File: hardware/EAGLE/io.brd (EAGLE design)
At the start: 17.8 x 110.5 mm, 23 parts, among them J10 PJ301_THONKICONN6, J11 PJ301_THONKICONN6, J12 PJ301_THONKICONN6, J13 PJ301_THONKICONN6, J2 PJ301_THONKICONN6, J3 PJ301_THONKICONN6, J4 PJ301_THONKICONN6, J5 PJ301_THONKICONN6, J6 PJ301_THONKICONN6, J7 PJ301_THONKICONN6, J8 PJ301_THONKICONN6, J9 PJ301_THONKICONN6

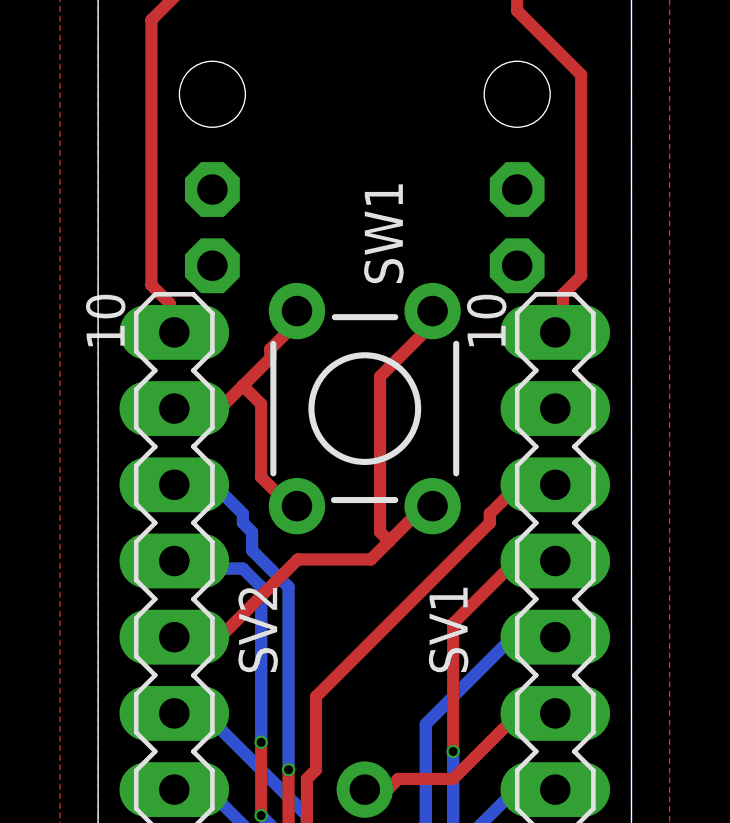
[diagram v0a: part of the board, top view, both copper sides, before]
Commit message: Submitted for Artist
and quick fixed layer errors
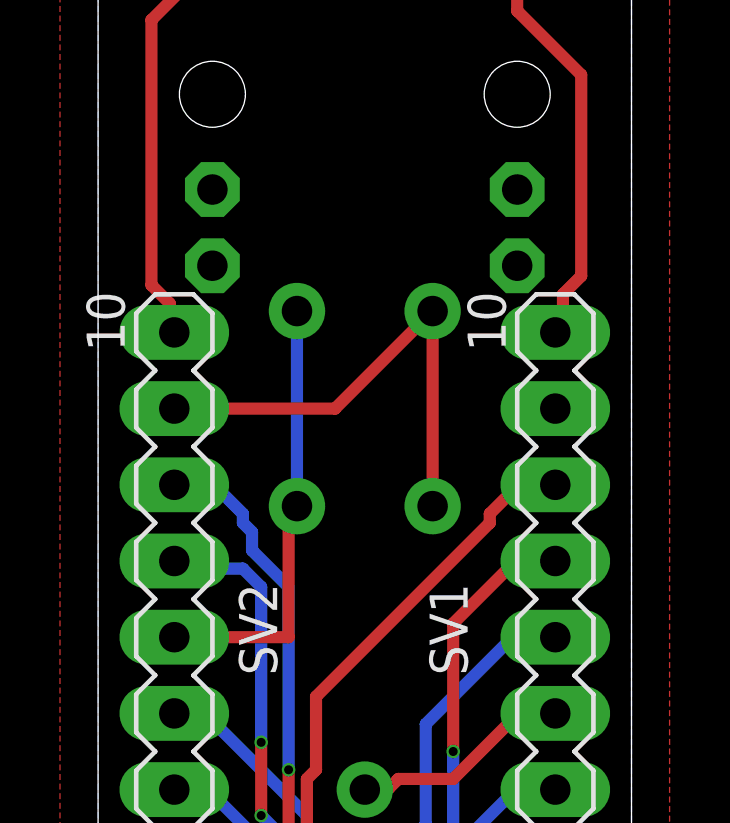
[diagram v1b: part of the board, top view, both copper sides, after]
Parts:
- flipped SW1 to the bottom
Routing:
- net +12V: track 10.8 -> 16.3 mm
- net BUTTON: track 19.1 -> 14.8 mm
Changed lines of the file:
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@@
 <attribute name="VALUE" x="13.97" y="14.351" size="1.27" layer="27" ratio="10" rot="R180"/>
 </element>
-<element name="SW1" library="SparkFun" package="TACTILE-PTH" value="" x="10.16" y="102.87" smashed="yes" rot="R90">
-<attribute name="NAME" x="10.16" y="110.49" size="1.27" layer="25" ratio="10" rot="R270"/>
+<element name="SW1" library="SparkFun" package="TACTILE-PTH" value="" x="10.16" y="102.87" smashed="yes" rot="MR90">
+<attribute name="NAME" x="10.16" y="110.49" size="1.27" layer="26" ratio="10" rot="MR270"/>
 </element>
 </elements>
@@
 <contactref element="SW1" pad="4"/>
 <contactref element="SW1" pad="3"/>
-<wire x1="5.4864" y1="95.4024" x2="3.9624" y2="95.4024" width="0.4064" layer="1"/>
-<wire x1="7.9248" y1="97.8408" x2="5.4864" y2="95.4024" width="0.4064" layer="1"/>
-<wire x1="10.3632" y1="97.8408" x2="7.9248" y2="97.8408" width="0.4064" layer="1"/>
-<wire x1="12.192" y1="99.6696" x2="10.9728" y2="98.4504" width="0.4064" layer="1"/>
-<wire x1="10.9728" y1="98.4504" x2="10.3632" y2="97.8408" width="0.4064" layer="1"/>
-<wire x1="3.9624" y1="95.4024" x2="3.81" y2="95.25" width="0.4064" layer="1"/>
-<wire x1="12.192" y1="99.6696" x2="12.4206" y2="99.6188" width="0.4064" layer="1"/>
-<wire x1="12.192" y1="105.4608" x2="12.192" y2="106.0704" width="0.4064" layer="1"/>
-<wire x1="10.668" y1="103.9368" x2="12.192" y2="105.4608" width="0.4064" layer="1"/>
-<wire x1="10.668" y1="98.7552" x2="10.668" y2="103.9368" width="0.4064" layer="1"/>
-<wire x1="10.9728" y1="98.4504" x2="10.668" y2="98.7552" width="0.4064" layer="1"/>
-<wire x1="12.192" y1="106.0704" x2="12.4206" y2="106.1212" width="0.4064" layer="1"/>
+<wire x1="7.8994" y1="99.6188" x2="7.62" y2="99.3394" width="0.4064" layer="1"/>
+<wire x1="7.62" y1="99.3394" x2="7.62" y2="95.25" width="0.4064" layer="1"/>
+<wire x1="7.62" y1="95.25" x2="3.81" y2="95.25" width="0.4064" layer="1"/>
+<wire x1="7.8994" y1="106.1212" x2="7.8994" y2="99.6188" width="0.4064" layer="16"/>
 </signal>
 <signal name="STEP">
@@
 <contactref element="SW1" pad="1"/>
 <contactref element="SW1" pad="2"/>
-<wire x1="5.4864" y1="103.0224" x2="3.9624" y2="103.0224" width="0.4064" layer="1"/>
-<wire x1="7.0104" y1="104.5464" x2="6.096" y2="103.632" width="0.4064" layer="1"/>
-<wire x1="6.096" y1="103.632" x2="5.4864" y2="103.0224" width="0.4064" layer="1"/>
-<wire x1="7.0104" y1="104.8512" x2="7.0104" y2="104.5464" width="0.4064" layer="1"/>
-<wire x1="7.62" y1="105.4608" x2="7.0104" y2="104.8512" width="0.4064" layer="1"/>
-<wire x1="7.62" y1="106.0704" x2="7.62" y2="105.4608" width="0.4064" layer="1"/>
-<wire x1="3.9624" y1="103.0224" x2="3.81" y2="102.87" width="0.4064" layer="1"/>
-<wire x1="7.62" y1="106.0704" x2="7.8994" y2="106.1212" width="0.4064" layer="1"/>
-<wire x1="6.7056" y1="100.584" x2="7.62" y2="99.6696" width="0.4064" layer="1"/>
-<wire x1="6.7056" y1="103.0224" x2="6.7056" y2="100.584" width="0.4064" layer="1"/>
-<wire x1="6.096" y1="103.632" x2="6.7056" y2="103.0224" width="0.4064" layer="1"/>
-<wire x1="7.62" y1="99.6696" x2="7.8994" y2="99.6188" width="0.4064" layer="1"/>
+<wire x1="12.4206" y1="106.1212" x2="12.2047" y2="105.9053" width="0.4064" layer="1"/>
+<wire x1="12.2047" y1="105.9053" x2="9.1694" y2="102.87" width="0.4064" layer="1"/>
+<wire x1="9.1694" y1="102.87" x2="3.81" y2="102.87" width="0.4064" layer="1"/>
+<wire x1="12.4206" y1="99.6188" x2="12.4206" y2="105.6894" width="0.4064" layer="1"/>
+<wire x1="12.4206" y1="105.6894" x2="12.2047" y2="105.9053" width="0.4064" layer="1"/>
 </signal>
 </signals>

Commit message: Added BOM
And buffer caps, and refined design
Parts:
- SV1, SV2: value (none) -> 1x10 pin header
- SV3: value (none) -> 1x3 pin header
- SW1: value (none) -> SPDT On-Off-On
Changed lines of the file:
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@@
 <layer number="25" name="tNames" color="7" fill="1" visible="yes" active="yes"/>
 <layer number="26" name="bNames" color="7" fill="1" visible="yes" active="yes"/>
-<layer number="27" name="tValues" color="7" fill="1" visible="no" active="yes"/>
-<layer number="28" name="bValues" color="7" fill="1" visible="no" active="yes"/>
-<layer number="29" name="tStop" color="7" fill="3" visible="no" active="yes"/>
-<layer number="30" name="bStop" color="7" fill="6" visible="no" active="yes"/>
-<layer number="31" name="tCream" color="7" fill="4" visible="no" active="yes"/>
-<layer number="32" name="bCream" color="7" fill="5" visible="no" active="yes"/>
-<layer number="33" name="tFinish" color="6" fill="3" visible="no" active="yes"/>
-<layer number="34" name="bFinish" color="6" fill="6" visible="no" active="yes"/>
-<layer number="35" name="tGlue" color="7" fill="4" visible="no" active="yes"/>
-<layer number="36" name="bGlue" color="7" fill="5" visible="no" active="yes"/>
-<layer number="37" name="tTest" color="7" fill="1" visible="no" active="yes"/>
-<layer number="38" name="bTest" color="7" fill="1" visible="no" active="yes"/>
+<layer number="27" name="tValues" color="7" fill="1" visible="yes" active="yes"/>
+<layer number="28" name="bValues" color="7" fill="1" visible="yes" active="yes"/>
+<layer number="29" name="tStop" color="7" fill="3" visible="yes" active="yes"/>
+<layer number="30" name="bStop" color="7" fill="6" visible="yes" active="yes"/>
+<layer number="31" name="tCream" color="7" fill="4" visible="yes" active="yes"/>
+<layer number="32" name="bCream" color="7" fill="5" visible="yes" active="yes"/>
+<layer number="33" name="tFinish" color="6" fill="3" visible="yes" active="yes"/>
+<layer number="34" name="bFinish" color="6" fill="6" visible="yes" active="yes"/>
+<layer number="35" name="tGlue" color="7" fill="4" visible="yes" active="yes"/>
+<layer number="36" name="bGlue" color="7" fill="5" visible="yes" active="yes"/>
+<layer number="37" name="tTest" color="7" fill="1" visible="yes" active="yes"/>
+<layer number="38" name="bTest" color="7" fill="1" visible="yes" active="yes"/>
 <layer number="39" name="tKeepout" color="4" fill="11" visible="yes" active="yes"/>
 <layer number="40" name="bKeepout" color="1" fill="11" visible="yes" active="yes"/>
 <layer number="41" name="tRestrict" color="4" fill="10" visible="yes" active="yes"/>
 <layer number="42" name="bRestrict" color="1" fill="10" visible="yes" active="yes"/>
-<layer number="43" name="vRestrict" color="2" fill="10" visible="no" active="yes"/>
-<layer number="44" name="Drills" color="7" fill="1" visible="no" active="yes"/>
-<layer number="45" name="Holes" color="7" fill="1" visible="no" active="yes"/>
-<layer number="46" name="Milling" color="3" fill="1" visible="no" active="yes"/>
-<layer number="47" name="Measures" color="7" fill="1" visible="no" active="yes"/>
-<layer number="48" name="Document" color="7" fill="1" visible="no" active="yes"/>
-<layer number="49" name="Reference" color="7" fill="1" visible="no" active="yes"/>
-<layer number="50" name="dxf" color="7" fill="1" visible="no" active="yes"/>
+<layer number="43" name="vRestrict" color="2" fill="10" visible="yes" active="yes"/>
+<layer number="44" name="Drills" color="7" fill="1" visible="yes" active="yes"/>
+<layer number="45" name="Holes" color="7" fill="1" visible="yes" active="yes"/>
+<layer number="46" name="Milling" color="3" fill="1" visible="yes" active="yes"/>
+<layer number="47" name="Measures" color="7" fill="1" visible="yes" active="yes"/>
+<layer number="48" name="Document" color="7" fill="1" visible="yes" active="yes"/>
+<layer number="49" name="Reference" color="7" fill="1" visible="yes" active="yes"/>
+<layer number="50" name="dxf" color="7" fill="1" visible="yes" active="yes"/>
 <layer number="51" name="tDocu" color="7" fill="1" visible="yes" active="yes"/>
 <layer number="52" name="bDocu" color="7" fill="1" visible="yes" active="yes"/>
@@
 <attribute name="VALUE" x="5.7785" y="78.74" size="0.6096" layer="28" font="vector" ratio="20" rot="MR270" align="top-center"/>
 </element>
-<element name="SV1" library="con-lstb" library_urn="urn:adsk.eagle:library:162" package="MA10-1" package3d_urn="urn:adsk.eagle:package:8346/1" value="" x="16.51" y="93.98" smashed="yes" rot="R90">
+<element name="SV1" library="con-lstb" library_urn="urn:adsk.eagle:library:162" package="MA10-1" package3d_urn="urn:adsk.eagle:package:8346/1" value="1x10 pin header" x="16.51" y="93.98" smashed="yes" rot="R90">
 <attribute name="MF" value="" x="16.51" y="93.98" size="1.778" layer="27" rot="R90" display="off"/>
 <attribute name="MPN" value="" x="16.51" y="93.98" size="1.778" layer="27" rot="R90" display="off"/>
@@
 <attribute name="VALUE" x="19.431" y="95.25" size="1.27" layer="27" ratio="10" rot="R90"/>
 </element>
-<element name="SV2" library="con-lstb" library_urn="urn:adsk.eagle:library:162" package="MA10-1" package3d_urn="urn:adsk.eagle:package:8346/1" value="" x="3.81" y="93.98" smashed="yes" rot="R90">
+<element name="SV2" library="con-lstb" library_urn="urn:adsk.eagle:library:162" package="MA10-1" package3d_urn="urn:adsk.eagle:package:8346/1" value="1x10 pin header" x="3.81" y="93.98" smashed="yes" rot="R90">
 <attribute name="MF" value="" x="3.81" y="93.98" size="1.778" layer="27" rot="R90" display="off"/>
 <attribute name="MPN" value="" x="3.81" y="93.98" size="1.778" layer="27" rot="R90" display="off"/>
@@
 <attribute name="VALUE" x="13.335" y="74.295" size="1.27" layer="27" rot="R180"/>
 </element>
-<element name="SV3" library="con-lstb" library_urn="urn:adsk.eagle:library:162" package="MA03-1" package3d_urn="urn:adsk.eagle:package:8339/1" value="" x="10.16" y="11.43" smashed="yes" rot="R180">
+<element name="SV3" library="con-lstb" library_urn="urn:adsk.eagle:library:162" package="MA03-1" package3d_urn="urn:adsk.eagle:package:8339/1" value="1x3 pin header" x="10.16" y="11.43" smashed="yes" rot="R180">
 <attribute name="MF" value="" x="10.16" y="11.43" size="1.778" layer="27" rot="R180" display="off"/>
 <attribute name="MPN" value="" x="10.16" y="11.43" size="1.778" layer="27" rot="R180" display="off"/>
@@
 <attribute name="VALUE" x="13.97" y="14.351" size="1.27" layer="27" ratio="10" rot="R180"/>
 </element>
-<element name="SW1" library="SparkFun" package="TACTILE-PTH" value="" x="10.16" y="102.87" smashed="yes" rot="MR90">
+<element name="SW1" library="SparkFun" package="TACTILE-PTH" value="SPDT On-Off-On" x="10.16" y="102.87" smashed="yes" rot="MR90">
 <attribute name="NAME" x="10.16" y="110.49" size="1.27" layer="26" ratio="10" rot="MR270"/>
 </element>
